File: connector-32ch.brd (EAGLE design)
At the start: 26.7 x 25.1 mm, 67 parts, among them X1 OMNETICS_36PAD

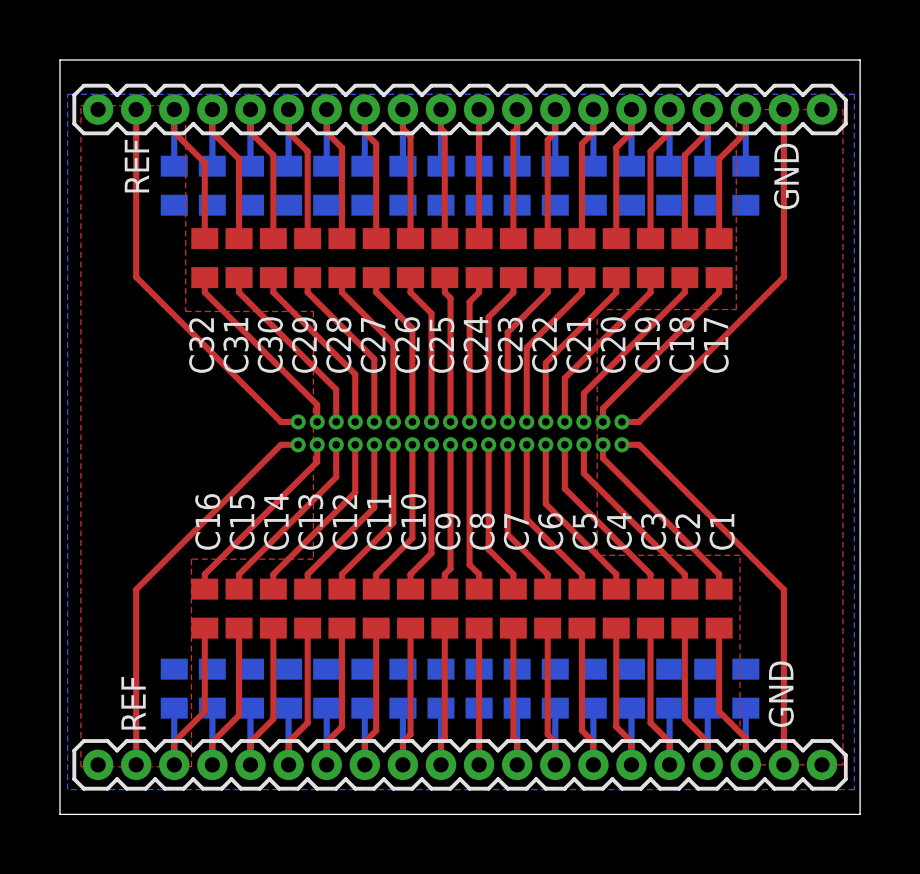
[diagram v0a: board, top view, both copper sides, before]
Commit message: almost final board files
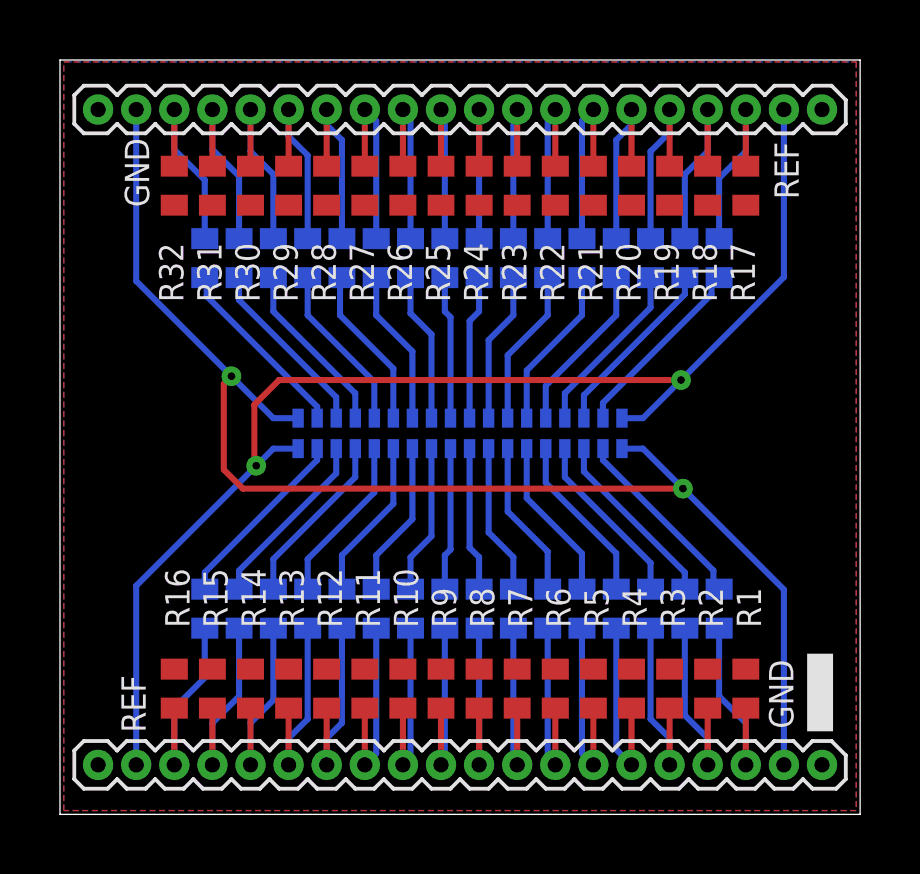
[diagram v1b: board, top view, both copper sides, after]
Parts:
- C1, C10, C11, C12, C13, C14, C15, C16, C17, C18, C19, C2, C20, C21, C22, C23, C24, C25, C26, C27, C28, C29, C3, C30, C31, C32, C4, C5, C6, C7, C8, C9: value (none) -> 22nf
- X1: device mor307:OMNETICS36PADPTH -> mor307:OMNETICS36PADSMT
- moved X1 0.63 mm to (13.3, 12.7)
- flipped C1 to the bottom
- flipped C10 to the bottom
- flipped C11 to the bottom
- flipped C12 to the bottom
- flipped C13 to the bottom
- flipped C14 to the bottom
- flipped C15 to the bottom
- flipped C16 to the bottom
- flipped C17 to the bottom
- flipped C18 to the bottom
- flipped C19 to the bottom
- flipped C2 to the bottom
- flipped C20 to the bottom
- flipped C21 to the bottom
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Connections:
- net G: now also JP1.2, X1.R1; no longer JP1.19, X1.G1
- net R: now also JP1.19, X1.G1; no longer JP1.2, X1.R1
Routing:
- net G: track 26.2 -> 45.0 mm, vias 0 -> 2
- net R: track 26.2 -> 42.8 mm, vias 0 -> 2
- added copper zone on layer 16, net G
- added copper zone on layer 1, net VCM
- removed copper zone on layer 1, net G
- removed copper zone on layer 1, net R
- removed copper zone on layer 16, net VCM
